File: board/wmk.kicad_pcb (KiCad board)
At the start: 4 copper layers, 34.5 x 100 mm, 26 parts, among them IC1 LM1117MPX-3.3, J1 Conn_01x03, U2 STM32F103C8T6, X1 PN87520-S

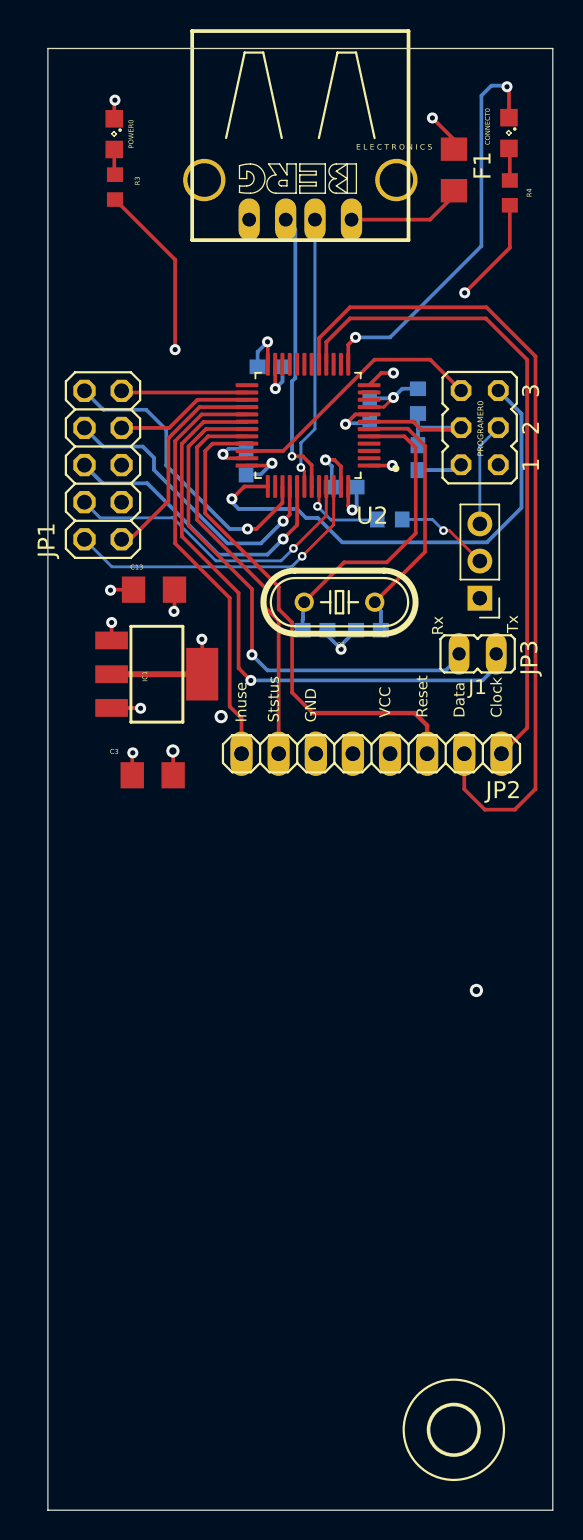
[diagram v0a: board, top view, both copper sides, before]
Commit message: gerbers
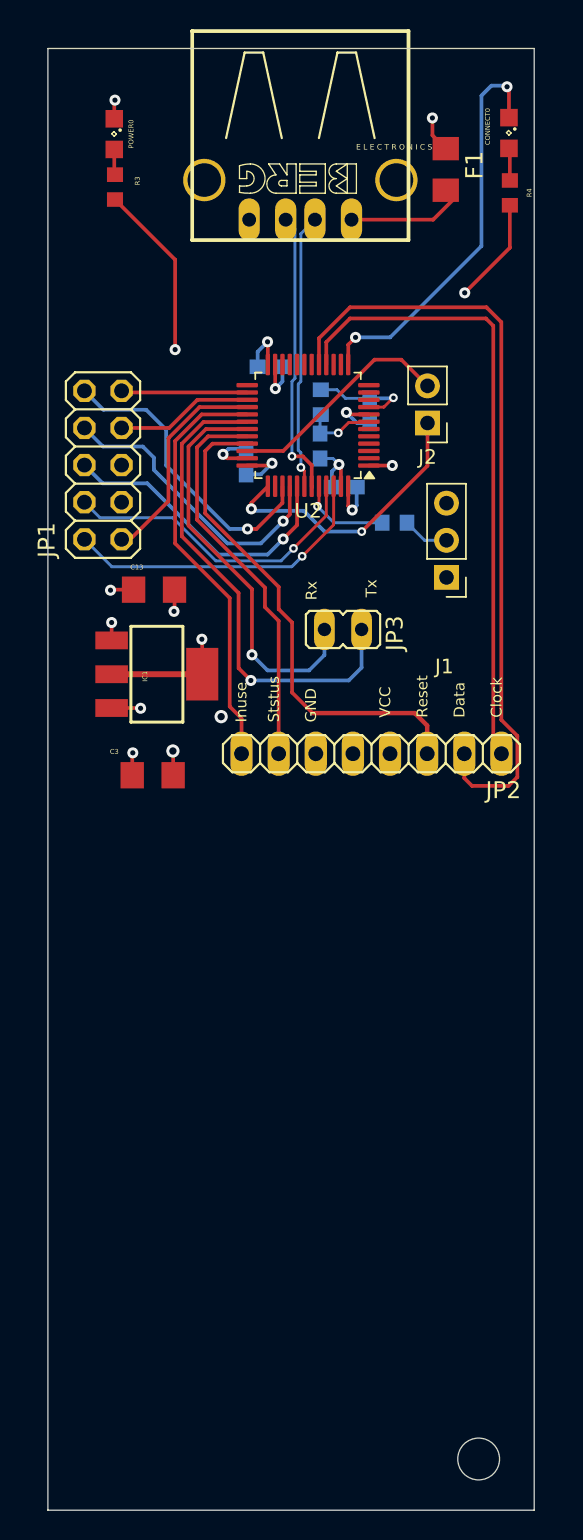
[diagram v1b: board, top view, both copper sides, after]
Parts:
- removed C10, C11: 22p, wmk:C0603
- removed PROGRAMER0: ~, wmk:JP3Q
- removed Q1: ~, wmk:HC49_S
- removed U$1: , wmk:3,3
- added J2: Conn_01x02, Connector_PinHeader_2.54mm:PinHeader_1x02_P2.54mm_Vertical, F.Cu at (157.2, 80.6)
- U2: footprint wmk:QFP50P900X900X160-48N -> Package_QFP:LQFP-48_7x7mm_P0.5mm
- moved JP3 9.36 mm to (151.4, 94.8)
- moved C7 6.74 mm to (149.8, 82.2)
- moved R2 6.65 mm to (149.9, 79.2)
- moved J1 2.69 mm to (158.5, 91.2)
- moved F1 0.56 mm to (158.4, 63.3)
- moved R1 0.40 mm to (154.9, 87.5)
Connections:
- U2 pad 5: Net-(U2-PD0_OSC_IN) -> unconnected-(U2-PD0_OSC_IN-Pad5)
- U2 pad 6: Net-(U2-PD1_OSC_OUT) -> unconnected-(U2-PD1_OSC_OUT-Pad6)
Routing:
- net Net-(U2-PD0_OSC_IN): track 20.9 -> 0.00 mm
- net Net-(U2-PD1_OSC_OUT): track 18.5 -> 0.00 mm
- net /SWCLK: track 33.6 -> 19.5 mm, vias 1 -> 2
- net /RX: track 36.8 -> 28.1 mm
- net /TX: track 42.3 -> 33.8 mm
- net /NRST: track 11.7 -> 5.01 mm, vias 0 -> 1
- net GND: track 27.4 -> 20.9 mm, vias 11 -> 9
- net VDD: track 54.4 -> 49.0 mm
- net /DATA: track 56.9 -> 52.9 mm
- net Net-(J1-Pin_2): track 6.49 -> 3.20 mm, vias 1 -> 0
- net /SWDIO: track 18.1 -> 15.7 mm
- net unconnected-(U2-PA2-Pad12): track 2.01 -> 0.00 mm, vias 1 -> 0
- net /CLOCK: track 44.8 -> 43.3 mm
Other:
- board size 34.5 x 100 mm -> 33.3 x 100 mm
